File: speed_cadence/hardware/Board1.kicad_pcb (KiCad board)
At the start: 2 copper layers, 8.6 x 5 mm, 10 parts, among them IC1 AH1912-W-7, J1 DX07S016JA3R1500, SW1 SW_Push, U1 STM32F042G6U6TR, U2 TS2940CW33_RPG

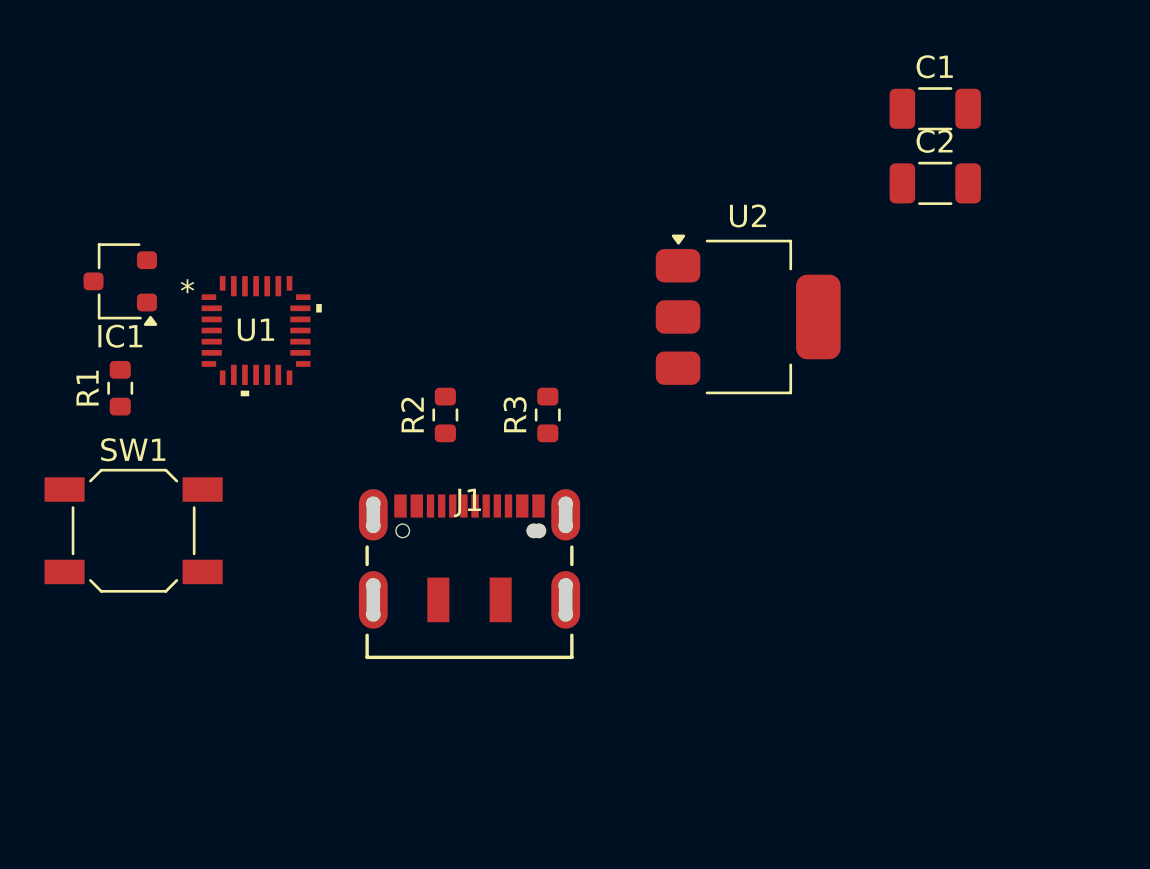
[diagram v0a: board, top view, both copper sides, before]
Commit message: Preliminary PCB placement
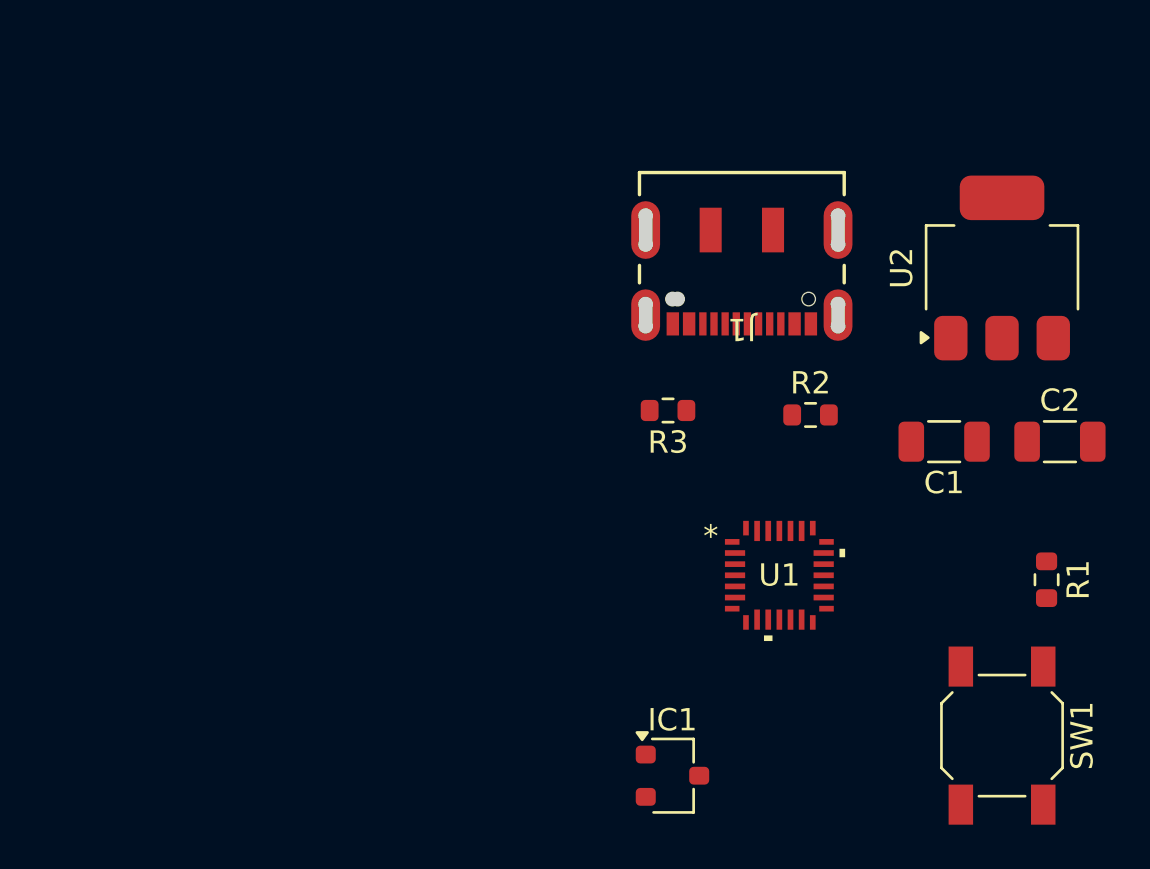
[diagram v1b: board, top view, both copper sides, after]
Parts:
- moved R1 42.5 mm to (95.0, 79.2), turned to -90 degrees
- moved SW1 40.1 mm to (93.0, 86.2), turned to -90 degrees
- moved IC1 33.3 mm to (78.2, 88.0), turned to 0 degrees
- moved U1 25.9 mm to (83.0, 79.0)
- moved J1 19.1 mm to (81.3, 64.5), turned to 180 degrees
- moved R2 16.4 mm to (84.4, 71.8), turned to 0 degrees
- moved C1 15.0 mm to (90.4, 73.0), turned to 180 degrees
- moved C2 12.9 mm to (95.6, 73.0)
- moved U2 11.6 mm to (93.0, 65.2), turned to 90 degrees
- moved R3 5.40 mm to (78.0, 71.6), turned to 180 degrees
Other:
- outline, holes or cut-outs redrawn
